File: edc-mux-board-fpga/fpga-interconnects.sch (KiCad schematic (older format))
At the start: 7 parts

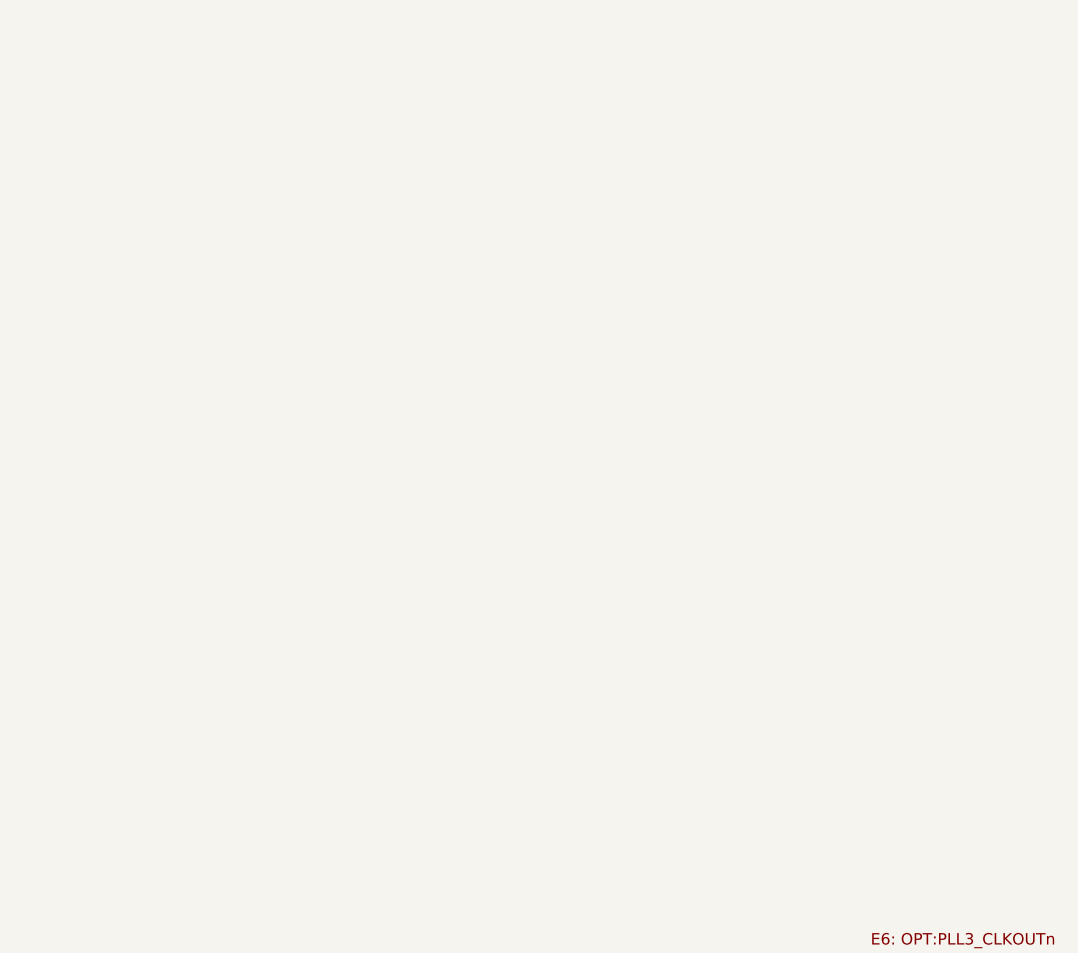
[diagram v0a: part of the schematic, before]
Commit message: starting to work on mezzanine board interconnections.
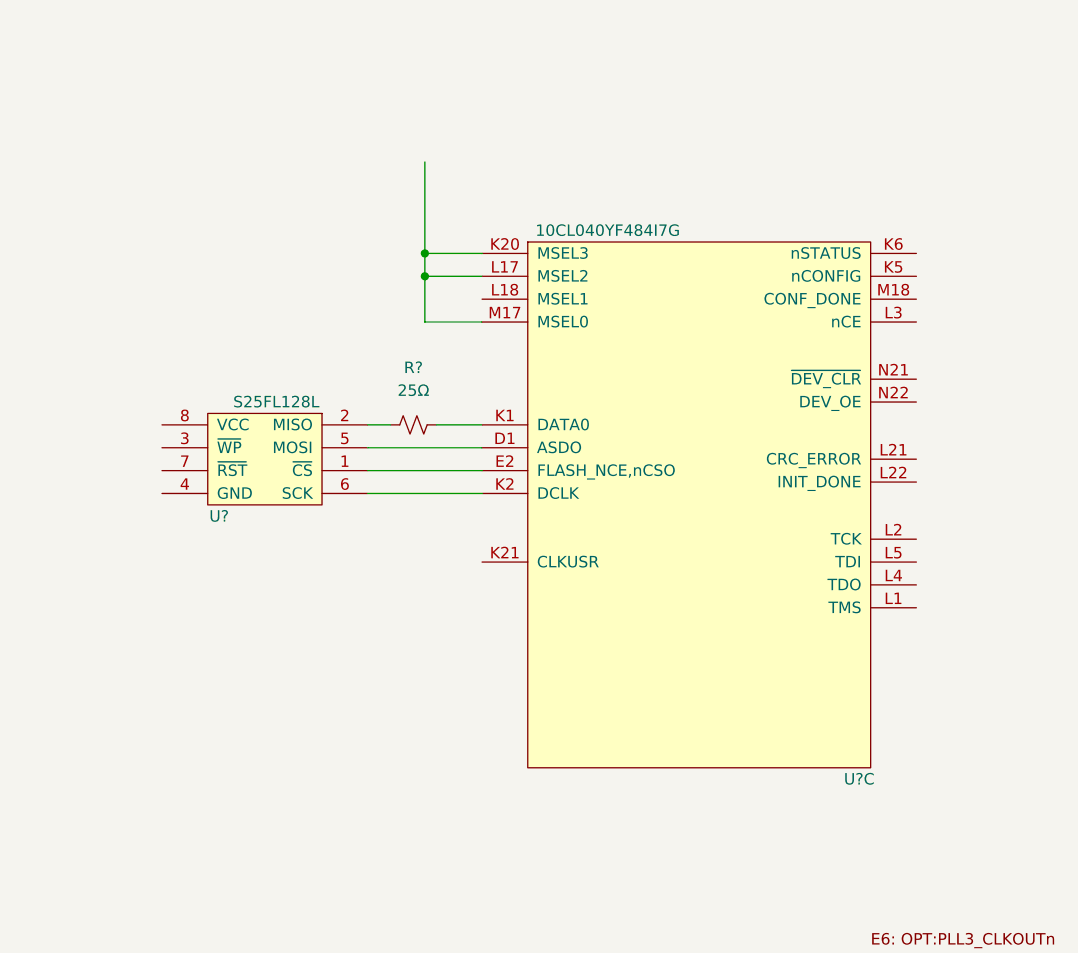
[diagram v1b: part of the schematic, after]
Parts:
- added R?: 25Ω, symbol Device:R_Small_US
- added U?: 10CL040YF484I7G, SW-Intel:FBGA-484_23.0x23.0mm_Layout22x22_P1.0mm, symbol SW-Intel:10CL040YF484I7G
- added U?: S25FL128L, symbol SW-Cypress:S25FL128L
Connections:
- wire segments 0 -> 11
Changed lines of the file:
@@
 $Descr USLedger 17000 11000
 encoding utf-8
-Sheet 22 25
+Sheet 25 28
 Title ""
 Date ""
@@
 AR Path="/5CC3E5DC/5CE97E21" Ref="U?"  Part="4"
 AR Path="/5CC6CC1A/5CD304E3/5CE97E21" Ref="U?"  Part="4"
+AR Path="/5CB2F6E3/5CE97E21" Ref="U?"  Part="4"
 F 0 "U?" H 15600 7800 50  0000 L CNN
 F 1 "10CL040YF484I7G" H 15600 7700 50  0000 L CNN
@@
 Text Label 5400 2300 0    50   ~ 0
 DIN2
+$Comp
+L SW-Intel:10CL040YF484I7G U?
+U 3 1 5CB19AD5
+P 9400 6500
+F 0 "U?" H 10100 5300 50  0000 C CNN
+F 1 "10CL040YF484I7G" H 9000 7700 50  0000 C CNN
+F 2 "SW-Intel:FBGA-484_23.0x23.0mm_Layout22x22_P1.0mm" H 12100 7400 50  0001 C CNN
+F 3 "https://www.intel.com/content/www/us/en/programmable/products/fpga/cyclone-series/cyclone-10/cyclone-10-lp/support.html" H 12100 7400 50  0001 C CNN
+	3    9400 6500
+	1    0    0    -1
+$EndComp
+$Comp
+L SW-Cypress:S25FL128L U?
+U 1 1 5CB411F7
+P 7500 6300
+F 0 "U?" H 7700 6050 50  0000 C CNN
+F 1 "S25FL128L" H 7450 6550 50  0000 C CNN
+F 2 "" H 7500 6300 50  0001 C CNN
+F 3 "https://www.cypress.com/file/316171/download" H 7500 6300 50  0001 C CNN
+	1    7500 6300
+	-1   0    0    -1
+$EndComp
+Wire Wire Line
+	7950 6150 8050 6150
+Wire Wire Line
+	7950 6450 8450 6450
+Wire Wire Line
+	7950 6350 8450 6350
+Wire Wire Line
+	7950 6250 8450 6250
+$Comp
+L Device:R_Small_US R?
+U 1 1 5CB55A13
+P 8150 6150
+F 0 "R?" V 7900 6150 50  0000 C CNN
+F 1 "25Ω" V 8000 6150 50  0000 C CNN
+F 2 "" H 8150 6150 50  0001 C CNN
+F 3 "~" H 8150 6150 50  0001 C CNN
+	1    8150 6150
+	0    1    1    0
+$EndComp
+Wire Wire Line
+	8250 6150 8450 6150
+Wire Wire Line
+	8450 5400 8200 5400
+Wire Wire Line
+	8200 5400 8200 5000
+Wire Wire Line
+	8450 5500 8200 5500
+Wire Wire Line
+	8200 5500 8200 5400
+Connection ~ 8200 5400
+Wire Wire Line
+	8450 5700 8200 5700
+Wire Wire Line
+	8200 5700 8200 5500
+Connection ~ 8200 5500
 $EndSCHEMATC
